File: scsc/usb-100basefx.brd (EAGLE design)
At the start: 44 x 44 mm, 59 parts, among them IC1 LD33, IC2 93LC66SN, U1 AX88772B, U2 AFBR-5803Z, Y1 25MHz

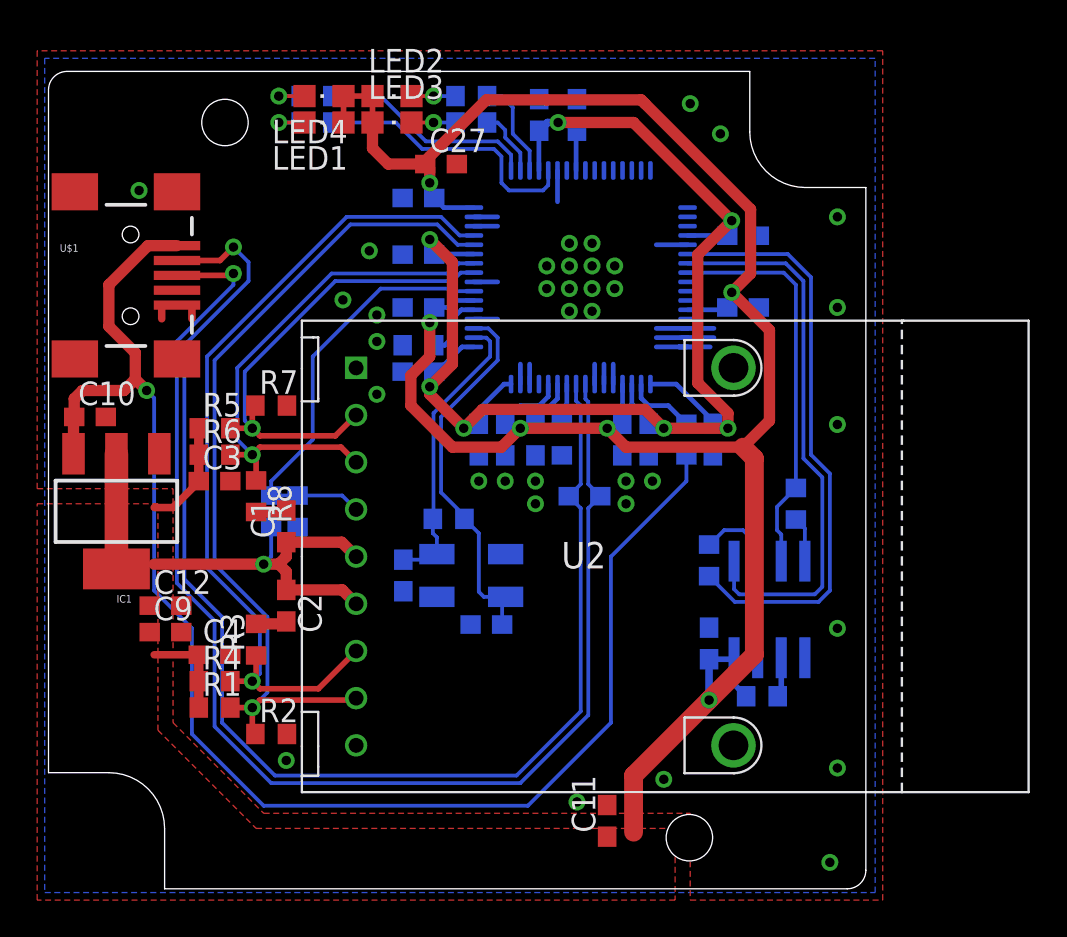
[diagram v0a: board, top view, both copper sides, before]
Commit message: hw: redone
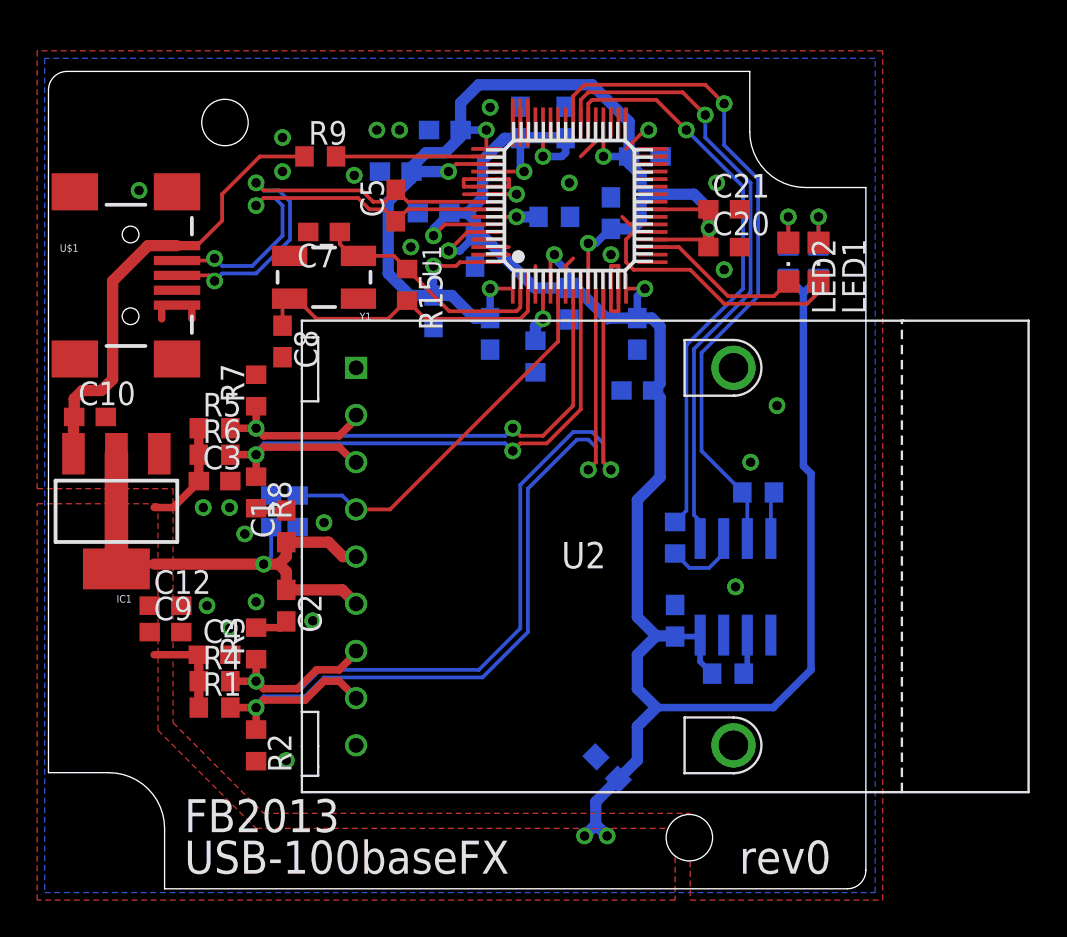
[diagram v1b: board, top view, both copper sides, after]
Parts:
- removed LED3, LED4: (no value), led:CHIPLED_0805
- removed R18, R19: 330, rcl:R0603
- U1: device balto:LQFP64 -> balto:LQFP64-0.4MM
- moved R16 28.1 mm to (41.5, 33.7), turned to 90 degrees
- moved LED1 27.7 mm to (41.5, 33.7), turned to 180 degrees
- moved R9 24.9 mm to (14.6, 39.4), flipped to the top, turned to 0 degrees
- moved LED2 23.1 mm to (39.8, 33.7), turned to 180 degrees
- moved C24 22.0 mm to (21.3, 40.8), turned to 0 degrees
- moved C23 19.8 mm to (18.7, 38.6), turned to 0 degrees
- moved R17 19.3 mm to (39.8, 33.7), turned to 90 degrees
- moved C7 19.0 mm to (14.8, 35.4), flipped to the top, turned to 180 degrees
- moved C8 18.8 mm to (12.6, 29.5), flipped to the top, turned to 270 degrees
- moved C5 18.7 mm to (18.7, 36.8), flipped to the top, turned to 90 degrees
- moved C14 17.9 mm to (25.4, 41.2), turned to 90 degrees
- moved Y1 17.9 mm to (14.8, 32.9), flipped to the top
- moved C27 16.1 mm to (31.7, 26.8), flipped to the bottom
- moved C18 13.9 mm to (31.7, 29.9), turned to 270 degrees
- moved C13 13.8 mm to (27.8, 41.2), turned to 90 degrees
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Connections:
- removed net LED3: R18.2, U1.18
- removed net LED4: R19.2, U1.17
- removed net N$10: LED4.C, R19.1
- removed net N$8: LED2.C, R17.1
- removed net N$9: LED3.C, R18.1
- new net N$6: LED1.A, R16.2
- net LED1: now also LED1.C; no longer R16.2
- net LED2: now also LED2.C; no longer R17.2
- net N$7: now also LED2.A, R17.2; no longer LED1.C, R16.1
- net VCC: now also R16.1, R17.1; no longer LED1.A, LED2.A, LED3.A, LED4.A
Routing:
- net USB_VIN: track 79.4 -> 24.7 mm, vias 1 -> 0
- net USB_DM: track 71.7 -> 23.3 mm, vias 1 -> 2
- net USB_DP: track 70.9 -> 24.8 mm, vias 1 -> 2
- net EE_DI: track 21.5 -> 36.7 mm, vias 0 -> 1
- net LED4: track 11.8 -> 0.00 mm
- net VDD: track 80.2 -> 69.9 mm
- net GND: track 30.4 -> 39.0 mm, vias 36 -> 26
- net RD_DP: track 26.4 -> 33.2 mm, vias 1 -> 2
- net VCC: track 158.5 -> 152.2 mm, vias 7 -> 9
- net RD_DN: track 28.8 -> 33.9 mm, vias 1 -> 2
- net N$1: track 3.77 -> 8.09 mm
- net TD_DN: track 46.0 -> 49.9 mm, vias 1 -> 2
- net EE_CS: track 30.1 -> 33.8 mm, vias 0 -> 1
- net LED3: track 3.66 -> 0.00 mm
- net LED2: track 5.41 -> 8.73 mm
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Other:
- board text added: "FB2013"
- board text added: "USB-100baseFX"
- board text added: "rev0"
